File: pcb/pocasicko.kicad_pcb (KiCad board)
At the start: 2 copper layers, 100 x 88 mm, 65 parts, among them J1 SMA, J2 Header_SMD_1x05, J3 FPC24, J4 Header_SMD_1x03, Q1 AO3400A, SW1 SW_Push, SW2 A, SW3 B, SW4 C, SW5 D, U1 CMWX1ZZABZ-091, U2 BME680, U3 MP28200, U4 LM66100

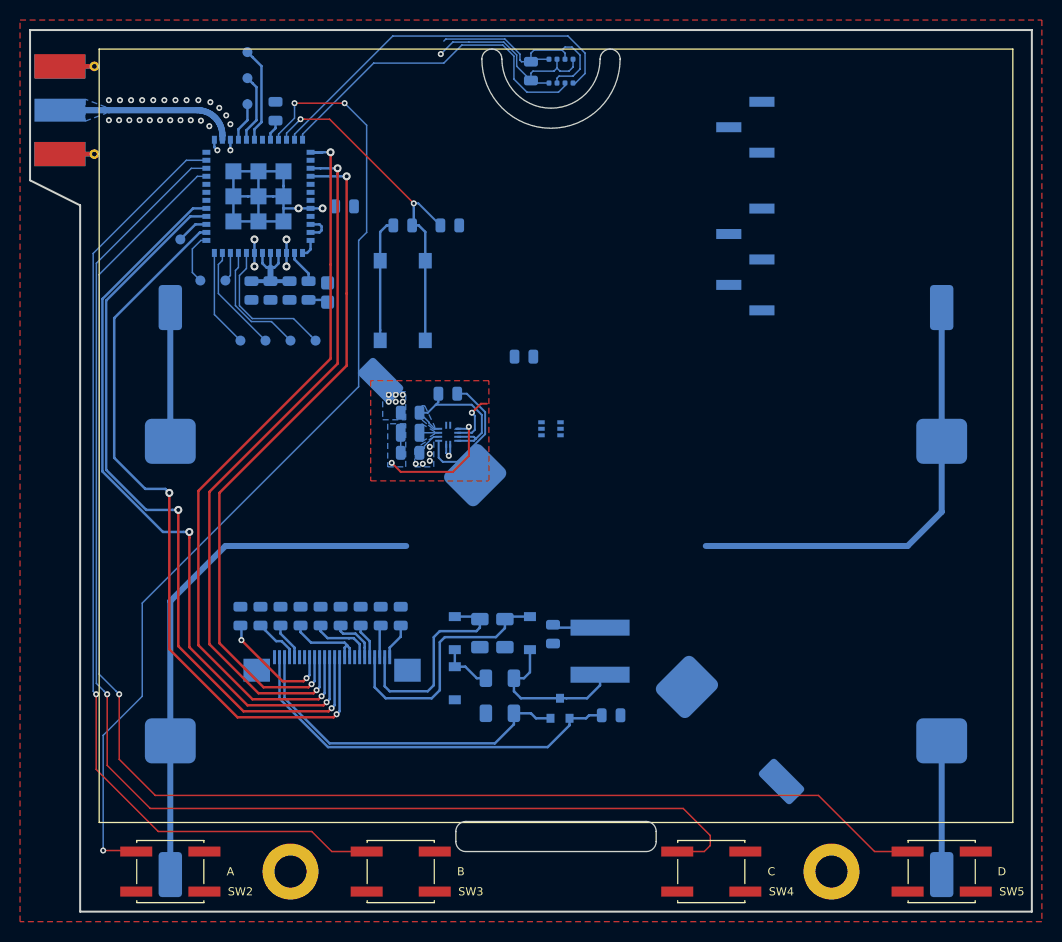
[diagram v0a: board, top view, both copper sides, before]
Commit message: Finished routing
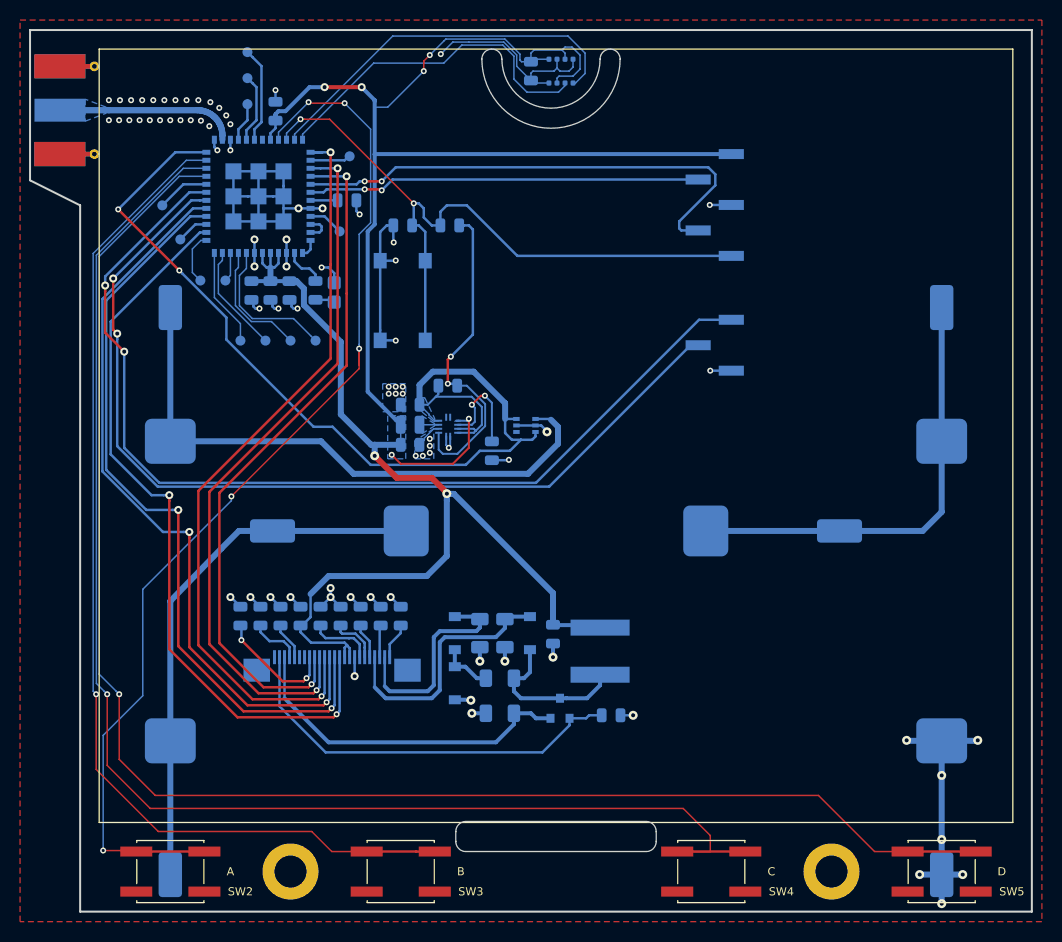
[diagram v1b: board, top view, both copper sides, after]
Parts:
- added TP11: PA8, TestPoint:TestPoint_Pad_D1.0mm, B.Cu at (113.2, 67.5)
- added TP12: PH1, TestPoint:TestPoint_Pad_D1.0mm, B.Cu at (130.9, 70.1)
- added TP13: PB7, TestPoint:TestPoint_Pad_D1.0mm, B.Cu at (131.9, 62.6)
- SW1: value SW_Push -> RESET
- moved J4 22.0 mm to (168.3, 81.5)
- moved R7 9.93 mm to (146.1, 92.0), turned to 90 degrees
- moved J2 6.24 mm to (168.3, 67.5)
- moved BT2 5.59 mm to (152.5, 100.0), turned to 0 degrees
- moved U4 2.52 mm to (149.5, 89.5)
- moved U3 0.80 mm to (141.7, 89.6)
- moved C2 0.80 mm to (137.9, 87.4)
- moved C6 0.80 mm to (137.9, 91.4)
- moved L1 0.80 mm to (137.9, 89.4)
- moved R3 0.80 mm to (141.7, 85.5)
- moved R2 0.69 mm to (128.5, 76.0)
- moved D3 0.67 mm to (130.4, 76.2)
- moved R1 0.65 mm to (131.6, 67.0)
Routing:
- net +2V5: track 64.7 -> 232.8 mm, vias 2 -> 8
- net /USART1_TX: track 0.00 -> 100.3 mm, vias 0 -> 2
- net /USART1_RX: track 0.00 -> 94.9 mm, vias 0 -> 2
- net /BATT_VOLTAGE: track 17.2 -> 101.8 mm, vias 0 -> 2
- net GND: track 93.2 -> 154.7 mm, vias 42 -> 81
- net /SWDIO: track 0.00 -> 50.3 mm, vias 0 -> 2
- net Net-(BT3-Pad1): track 13.3 -> 58.9 mm
- net /SWCLK: track 0.00 -> 39.3 mm, vias 0 -> 2
- net /~MCU_RESET: track 35.7 -> 68.9 mm
- net /POWER_GOOD: track 13.4 -> 32.4 mm, vias 0 -> 2
- net /BUTTON_D: track 146.5 -> 154.4 mm
- net /BUTTON_A: track 99.1 -> 106.7 mm, vias 3 -> 5
- net /BUTTON_C: track 133.1 -> 140.7 mm
- net /BUTTON_B: track 97.2 -> 104.0 mm
- net Net-(TP11-Pad1): track 0.00 -> 5.27 mm
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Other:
- board text removed: "Bačísek"
- board text removed: "Chookity!"
- board text removed: "Is it Tribore? Yes, it is!"
